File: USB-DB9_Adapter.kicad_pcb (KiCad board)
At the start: 2 copper layers, 31.8 x 32.1 mm, 33 parts, among them IC2 STM32G0B1KBU6-N, X1 USB-1X-2S-PLUG-A-SMD, X7 SWD_MOSER_CONN_5_POLST

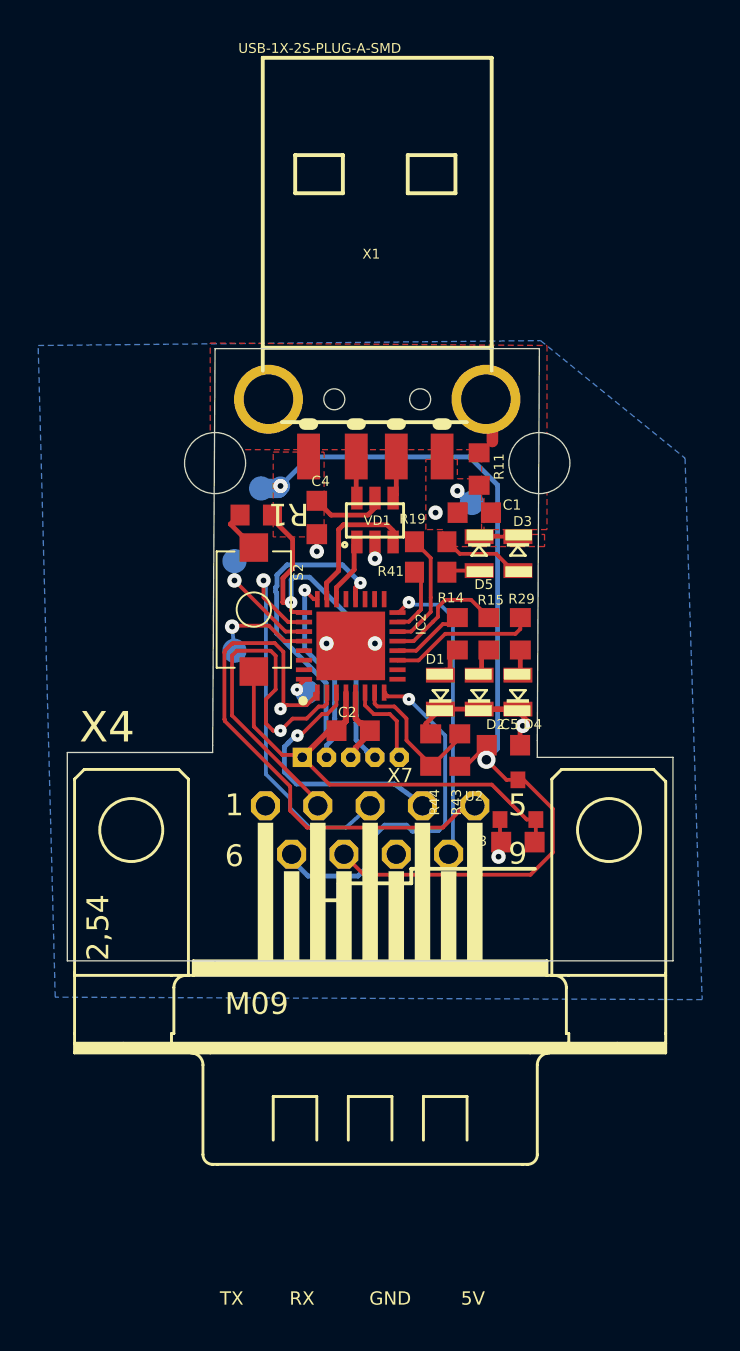
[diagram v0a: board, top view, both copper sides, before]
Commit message: Add files via upload
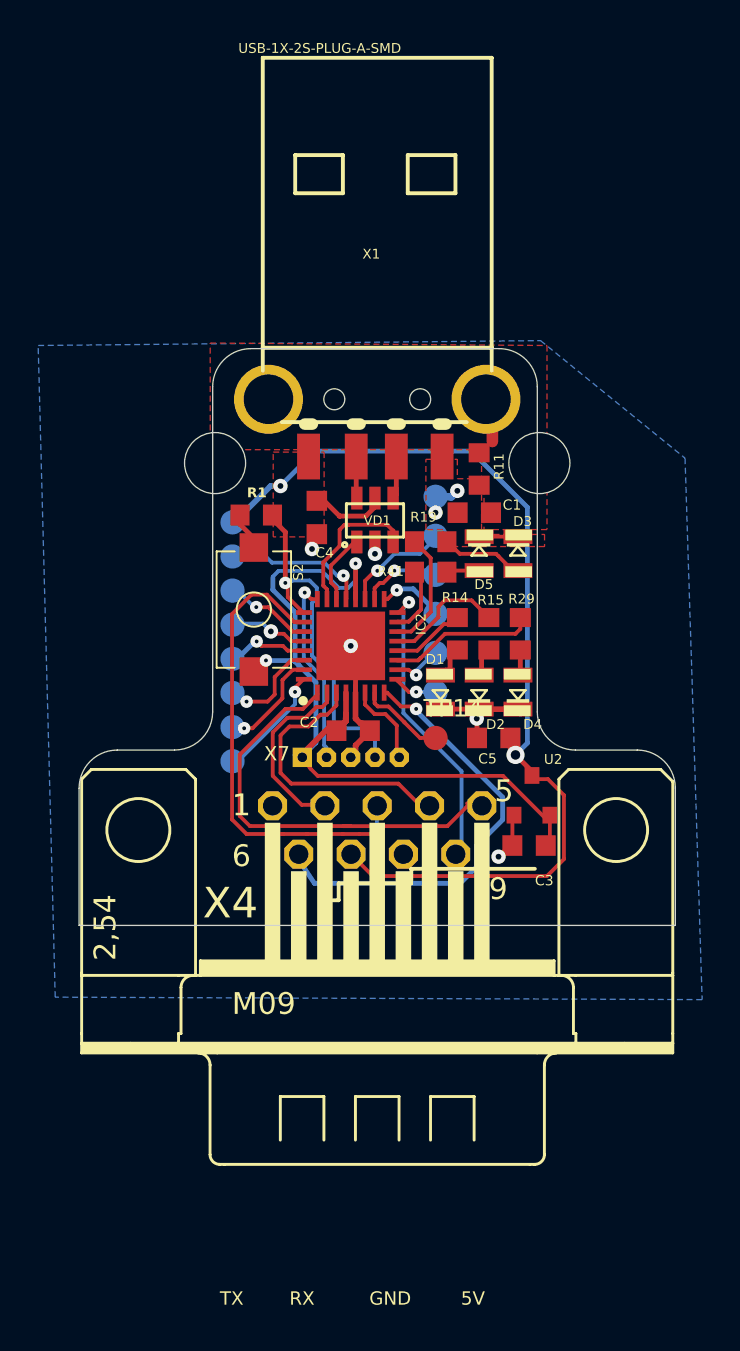
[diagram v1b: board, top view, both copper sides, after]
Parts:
- removed R43: 200K, 0603
- removed R44: 40.2K, 0603
- added TP1: don't show, TESTPUNKT, B.Cu at (141.1, 108.9)
- added TP12: don't show, TESTPUNKT, B.Cu at (151.9, 103.5)
- added TP13: don't show, TESTPUNKT, B.Cu at (141.4, 99.7)
- added TP14: don't show, TESTPUNKT, F.Cu at (151.9, 109.4)
- added TP15: don't show, TESTPUNKT, B.Cu at (141.1, 105.0)
- added TP2: don't show, TESTPUNKT, B.Cu at (141.3, 107.0)
- added TP4: don't show, TESTPUNKT, B.Cu at (151.9, 105.2)
- added TP7: don't show, TESTPUNKT, B.Cu at (151.9, 107.0)
- added TP8: don't show, TESTPUNKT, B.Cu at (151.9, 99.0)
- added TP9: don't show, TESTPUNKT, B.Cu at (151.9, 100.6)
- moved TP3 5.45 mm to (141.1, 110.6)
- moved TP10 2.11 mm to (141.7, 98.1)
- moved TP11 1.93 mm to (151.9, 96.7)
- moved TP5 1.66 mm to (141.3, 103.1)
- moved TP6 1.40 mm to (141.3, 101.5)
- moved U2 0.77 mm to (157.0, 112.3)
- moved C5 0.63 mm to (155.0, 109.4), turned to 180 degrees
- moved C3 0.61 mm to (156.8, 115.0)
- moved X4 0.37 mm to (148.9, 114.2)
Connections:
- IC2 pad 10: (no net) -> N$5
- IC2 pad 17: (no net) -> N$15
- IC2 pad 18: (no net) -> N$14
- IC2 pad 19: (no net) -> N$13
- IC2 pad 21: (no net) -> N$16
- IC2 pad 30: (no net) -> N$10
- IC2 pad 31: (no net) -> N$11
- IC2 pad 9: (no net) -> N$9
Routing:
- net DOWN: track 20.6 -> 9.30 mm, vias 1 -> 0
- net N$16: track 0.00 -> 7.49 mm, vias 0 -> 1
- net BUTTON3: track 29.4 -> 22.5 mm, vias 1 -> 0
- net N$11: track 0.00 -> 5.86 mm, vias 0 -> 1
- net N$13: track 0.00 -> 5.76 mm, vias 0 -> 1
- net N$10: track 0.00 -> 5.36 mm, vias 0 -> 1
- net N$15: track 0.00 -> 4.82 mm, vias 0 -> 1
- net N$19: track 0.00 -> 4.63 mm, vias 0 -> 1
- net LEFT: track 21.1 -> 25.7 mm
- net N$39: track 1.70 -> 6.15 mm
- net N$14: track 0.00 -> 4.08 mm, vias 0 -> 1
- net BUTTON1: track 19.7 -> 23.6 mm
- net N$44: track 7.95 -> 4.51 mm
- net N$5: track 0.00 -> 2.71 mm, vias 0 -> 1
- net N$9: track 0.00 -> 2.31 mm, vias 0 -> 1
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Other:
- board size 31.8 x 32.1 mm -> 31.3 x 30.2 mm
- board text added: "USB-DB9 Adapter by M.& S. Beha"
- board text removed: "USB-DB9 Adapter"

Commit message: Add files via upload
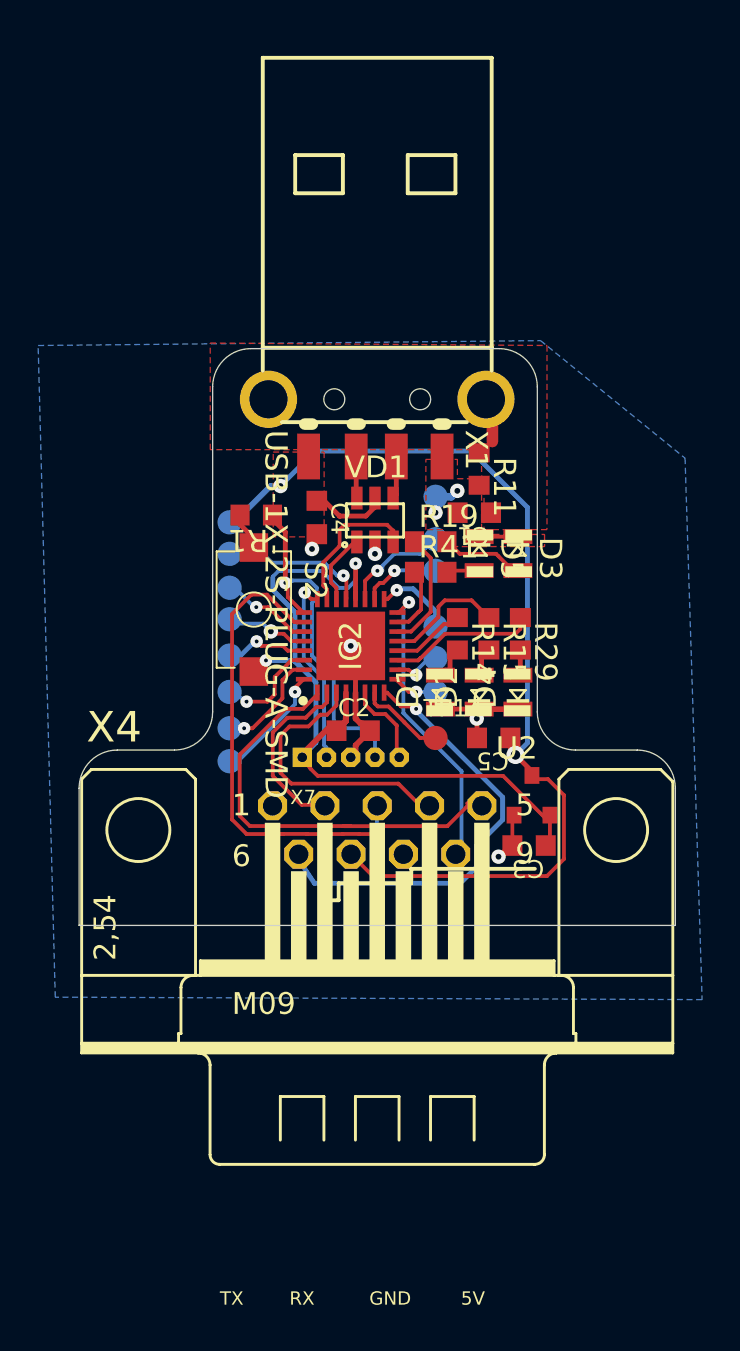
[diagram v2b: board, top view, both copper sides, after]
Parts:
- removed UNK_HOLE_0: , dummyfp0
- removed UNK_HOLE_1: , dummyfp1
- C1, C2, C3, C4, C5: footprint C0603 -> USB-DB9_Adapter:C0603
- D1, D2, D3, D4, D5: footprint 0805_D -> USB-DB9_Adapter:0805_D
- IC2: footprint QFN50P500X500X60-33N -> USB-DB9_Adapter:QFN50P500X500X60-33N
- R1, R11, R14, R15, R19, R29, R41: footprint 0603 -> USB-DB9_Adapter:0603
- S2: value (none) -> TASER_KSR; footprint KSR_TASTER -> USB-DB9_Adapter:KSR_TASTER
- TP1, TP10, TP11, TP12, TP13, TP14, TP15, TP2, TP3, TP4, TP5, TP6, TP7, TP8, TP9: footprint TESTPUNKT -> USB-DB9_Adapter:TESTPUNKT
- U2: value (none) -> U_SPANNUNGSREGLERSOT23; footprint SOT23 -> USB-DB9_Adapter:SOT23
- VD1: footprint SOT-23-6L -> USB-DB9_Adapter:SOT-23-6L
- X1: footprint USB-PLUG-A-SMD-2S -> USB-DB9_Adapter:USB-PLUG-A-SMD-2S
- X4: value (none) -> M09H; footprint M09H -> USB-DB9_Adapter:M09H
- X7: footprint SWD_MOSER_CONN_5_POL_.5MM -> USB-DB9_Adapter:SWD_MOSER_CONN_5_POL_.5MM
- moved TP10 0.51 mm to (141.1, 98.1)
- moved TP13 0.25 mm to (141.1, 99.7)
- moved TP2 0.13 mm to (141.1, 107.0)
- moved TP5 0.13 mm to (141.1, 103.1)
- moved TP6 0.13 mm to (141.1, 101.5)
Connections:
- net 3V3 renamed /3V3
- net BUTTON1 renamed /BUTTON1
- net BUTTON2 renamed /BUTTON2
- net BUTTON3 renamed /BUTTON3
- net DM renamed Net-(IC2-PA11_[PA9])
- net DOWN renamed /DOWN
- net DP renamed Net-(IC2-PA12_[PA10])
- net LEFT renamed /LEFT
- net MISO renamed Net-(IC2-PA4)
- net RIGHT renamed /RIGHT
- net SCK renamed Net-(IC2-PA5)
- net SHIELD renamed Net-(C1-Pad1)
- net UP renamed /UP
